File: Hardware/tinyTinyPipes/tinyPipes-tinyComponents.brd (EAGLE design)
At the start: 59 x 59 mm, 112 parts, among them Q1 CJ2302, Q2 IRFR5305, Q3 CJ2302, Q5 S9013, Q6 S9013, Q7 S9013, U1 TD1410, U2 ICS_V54_SIM900, U3 ATMEGA168, U4 MAX4372, U5 SI4435POWER, U6 MAX4372, U7 EEPROM-I2CSMD

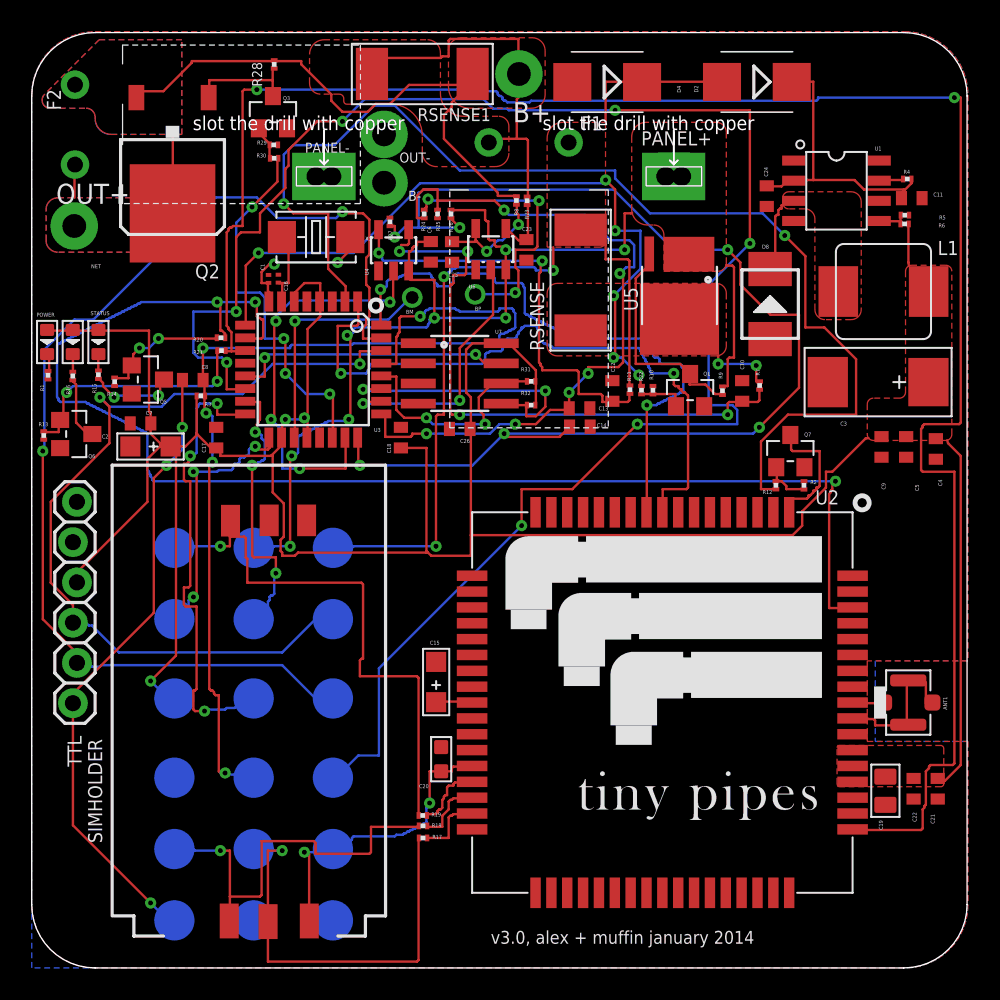
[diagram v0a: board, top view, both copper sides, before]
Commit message: pushing up tinyComponents PCB and various firmware changes
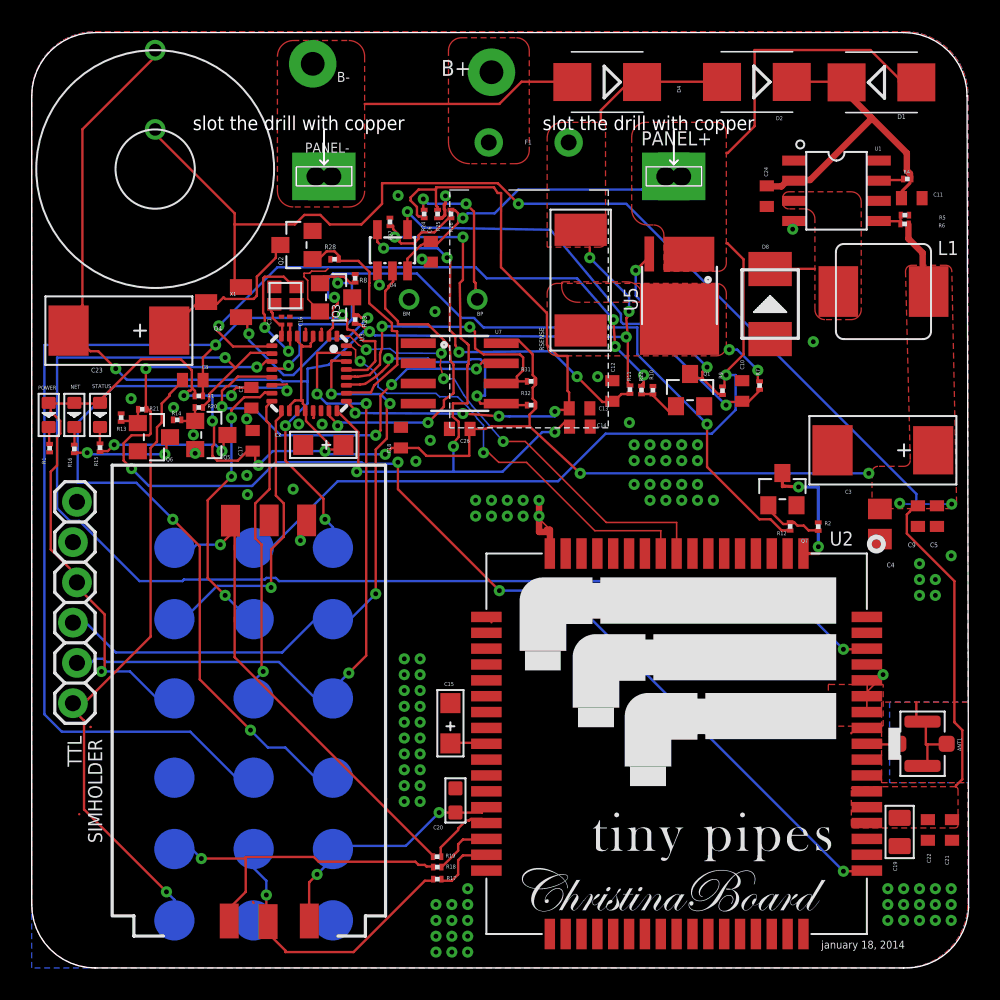
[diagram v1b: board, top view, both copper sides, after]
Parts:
- removed C25: 100nF, rcl:C0402
- removed F2: (no value), tinyPipes v2.6:0210
- removed OUT+, OUT-: TINYPIPES_BATTBATT, tinyPipes v2.6:TINYPIPES_BATT
- removed R29: 100k, rcl:R0201
- removed R30: 1k, rcl:R0201
- removed RSENSE1: 0.003, 1%, Discrete:R2512
- removed U6: MAX4372, tinyPipes:SOT23-5
- added D1: SS54, diode:SMB
- added Q4: BSS84, transistor-small-signal:SOT23
- added U$1: INDUCTOR, tinyPipes:10UH_5A_INDUCTOR
- C23: value 100nF -> 470uF 6.3V; device rcl:C0402 -> Discrete:AVX-D
- C4: value 10uF -> 10uF; device rcl:C0402 -> rcl:C0805
- Q2: value IRFR5305 -> CJ2302; device transistor-power:D-PAK_TO252AA -> Discrete:SOT23
- U3: value ATMEGA168 -> ATMEGA168MLF; device SparkFun:TQFP32-08 -> tinyPipes:MLF32
- X1: value (none) -> 16mhz; device Discrete:2P-SMD-5X3.2 -> tinyPipes:SMD-4_CRYSTAL
- moved C23 26.2 mm to (5.50, 40.2), turned to 180 degrees
- moved R23 13.2 mm to (20.4, 40.9)
- moved R28 12.9 mm to (19.1, 44.7), turned to 0 degrees
- moved Q3 12.3 mm to (19.2, 42.3), turned to 270 degrees
- moved R8 11.3 mm to (20.4, 43.5)
- moved C2 10.9 mm to (18.4, 33.0)
- moved Q2 9.02 mm to (16.7, 45.6), turned to 90 degrees
- moved B- 8.75 mm to (17.7, 57.0)
- moved C7 7.17 mm to (13.9, 36.0), turned to 90 degrees
- moved R21 6.22 mm to (6.97, 35.2)
- moved C4 5.91 mm to (53.5, 28.0), turned to 270 degrees
- moved Q5 5.32 mm to (11.3, 33.6)
- moved R13 5.01 mm to (5.64, 34.7), turned to 270 degrees
- moved C9 4.93 mm to (55.9, 28.5), turned to 270 degrees
- moved Q6 4.90 mm to (7.71, 33.5)
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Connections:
- removed net BATTERY_CURRENT: U3.26, U6.2
- removed net BATT_EN: R30.2, U3.22
- removed net DEK: Q2.3, R28.2, R8.1, RSENSE1.1
- removed net N$14: C25.2, R8.2, U6.5
- removed net N$18: F2.2, Q2.4
- removed net N$19: F2.1, OUT+.1
- removed net N$20: Q2.1, Q3.3, R28.1
- removed net N$21: Q3.1, R29.2, R30.1
- removed net N$23: B+.1, F1.1, R23.1, RSENSE1.2
- new net B+: B+.1, F1.1
- new net B-: B-.1, D4.A
- new net HIGH_SIDE: Q3.1, R8.2, U3.12
- new net LOW_SIDE: Q2.1, R28.2, U3.26
- new net PFET_GATE: Q3.3, Q4.1, R23.1
- new net VROUTE: C17.2, C18.2, C19.2, C2.+, C21.2, C22.2, C26.1, C3.+, C4.1, C5.1, C7.2, C9.1, L1.2, NETLIGHT.+, POWER.+, R3.2, R31.2, R32.2, R6.2, STATUS.+, TTL.4, U2.55, U2.56, U2.57, U3.18, U3.20, U3.4, U3.6, U7.8, VCC.TP
- net BATTERY: now also C23.-, R23.2, U$1.P$2
- net BV-: no longer U3.19
- net GND: now also C4.2, C5.2, C9.2, Q2.2, R28.1, R8.1; no longer B-.1, C23.2, C25.1, C4.1, C5.1, C9.1, D4.A, OUT-.1, R29.1, U6.1
- net N$17: now also C23.+, Q2.3, Q4.3; no longer C23.1, R23.2, U6.4
- net N$2: now also X1.3; no longer X1.2
- net PANEL: now also D1.A; no longer U6.3
- net VCC: now also Q4.2, U$1.P$1; no longer C17.2, C18.2, C19.2, C2.+, C21.2, C22.2, C26.1, C3.+, C4.2, C5.2, C7.2, C9.2, L1.2, NETLIGHT.+, POWER.+, R3.2, R31.2, R32.2, R6.2, STATUS.+, TTL.4, U2.55, U2.56, U2.57, U3.18, U3.20, U3.4, U3.6, U7.8, VCC.TP
- net VDD: now also D1.C
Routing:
- net VROUTE: track 0.00 -> 134.6 mm, vias 0 -> 9
- net VCC: track 171.5 -> 70.2 mm
- net LOAD_FET: track 115.3 -> 48.2 mm, vias 7 -> 3
- net NETLIGHT: track 121.2 -> 75.5 mm, vias 2 -> 6
- net BATTERY: track 54.9 -> 91.4 mm, vias 3 -> 7
- net DEK: track 36.4 -> 0.00 mm
- net PANEL_VOLTAGE: track 77.3 -> 45.8 mm, vias 6 -> 5
- net GSM_POWER: track 73.3 -> 42.9 mm
- net TX: track 72.4 -> 44.9 mm, vias 2 -> 3
- net N$23: track 24.0 -> 0.00 mm
- net BATT_EN: track 23.7 -> 0.00 mm, vias 4 -> 0
- net PANEL: track 66.1 -> 87.0 mm, vias 8 -> 2
- net BATTERY_CURRENT: track 16.6 -> 0.00 mm, vias 2 -> 0
- net GND: track 9.03 -> 24.5 mm, vias 0 -> 107
- net BV-: track 15.4 -> 0.00 mm, vias 1 -> 0
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- added copper zone on layer 1, net B+
- added copper zone on layer 1, net B-
- added copper zone on layer 1, net VROUTE
- removed copper zone on layer 1, net BATT
- removed copper zone on layer 1, net N$10
- removed copper zone on layer 1, net N$18
- removed copper zone on layer 16, net N$18
- removed copper zone on layer 1, net N$19
- removed copper zone on layer 16, net N$19
- removed copper zone on layer 1, net VCC
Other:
- board size 59 x 59 mm -> 59.1 x 59 mm
- board text added: "january 18, 2014"
- board text removed: "v3.0, alex + muffin january 2014"
